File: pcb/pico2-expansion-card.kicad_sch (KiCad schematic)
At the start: 50 parts, among them J3 Conn_01x03_Socket, J4 Conn_01x04_Socket, Q1 EM6K6, Q2 EM6K6, SW1 SW_Push, U2 RP2354A, U4 AP2127K-3.3, Y1 ABM8-272-T3

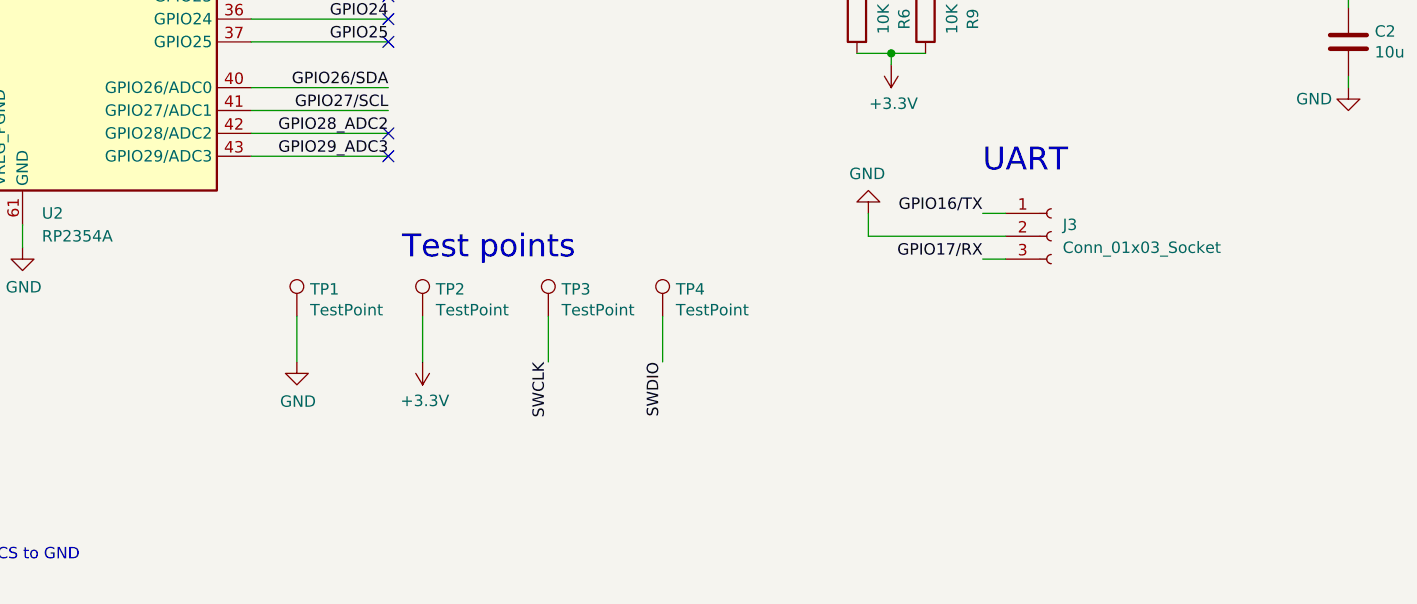
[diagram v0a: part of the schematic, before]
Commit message: fix false UART
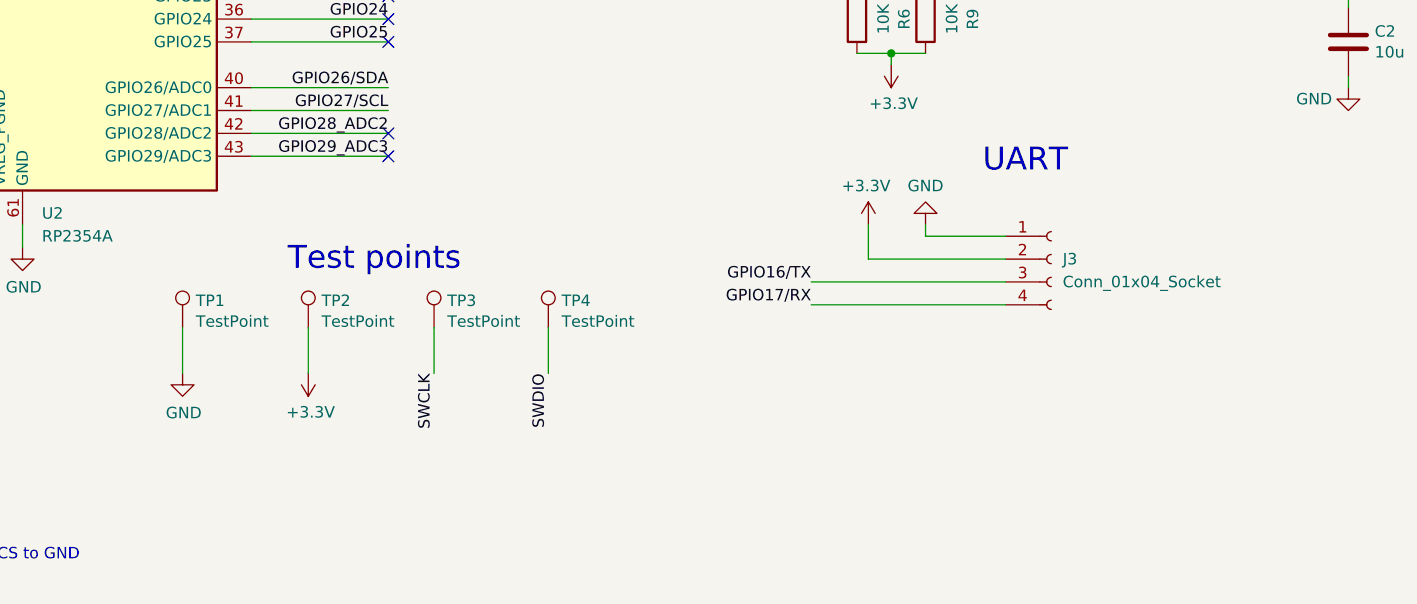
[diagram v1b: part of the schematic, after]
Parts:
- removed J3: Conn_01x03_Socket, Connector_JST:JST_SH_SM03B-SRSS-TB_1x03-1MP_P1.00mm_Horizontal, symbol Connector:Conn_01x03_Socket
- added J3: Conn_01x04_Socket, Connector_JST:JST_SH_SM04B-SRSS-TB_1x04-1MP_P1.00mm_Horizontal, symbol Connector:Conn_01x04_Socket
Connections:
- net +3.3V: now also J3.2 (Pin_2)
- net GND: now also J3.1 (Pin_1)
- net GPIO16/TX: now also J3.3 (Pin_3)
- net GPIO17/RX: now also J3.4 (Pin_4)
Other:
- moved on the sheet: TP1, TP2, TP3, TP4
